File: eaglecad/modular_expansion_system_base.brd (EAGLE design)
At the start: 90.2 x 100 mm, 36 parts, among them IC1 74LS244N, IC2 74LS244N, IC3 74LS244N, IC4 SRAM, IC5 74LS30N, IC6 74LS30N, IC7 7805T, IC8 74LS00N, IC9 7805T, J1_ADDRESS_CON j1, J2_DATA_AND_POWER_CON j2, J3 interrupt_wait_block, SW1 100SP3T1B1M6QE

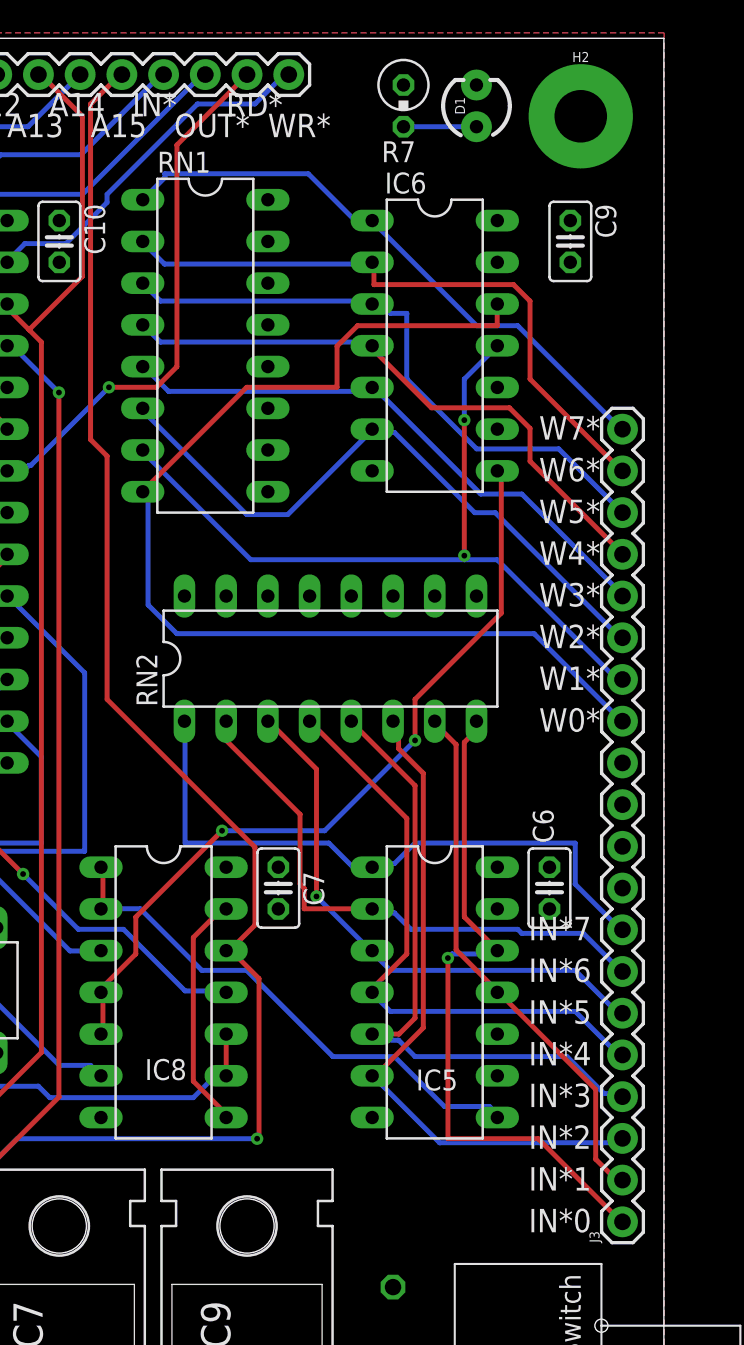
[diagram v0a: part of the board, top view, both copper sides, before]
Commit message: all three boards designed
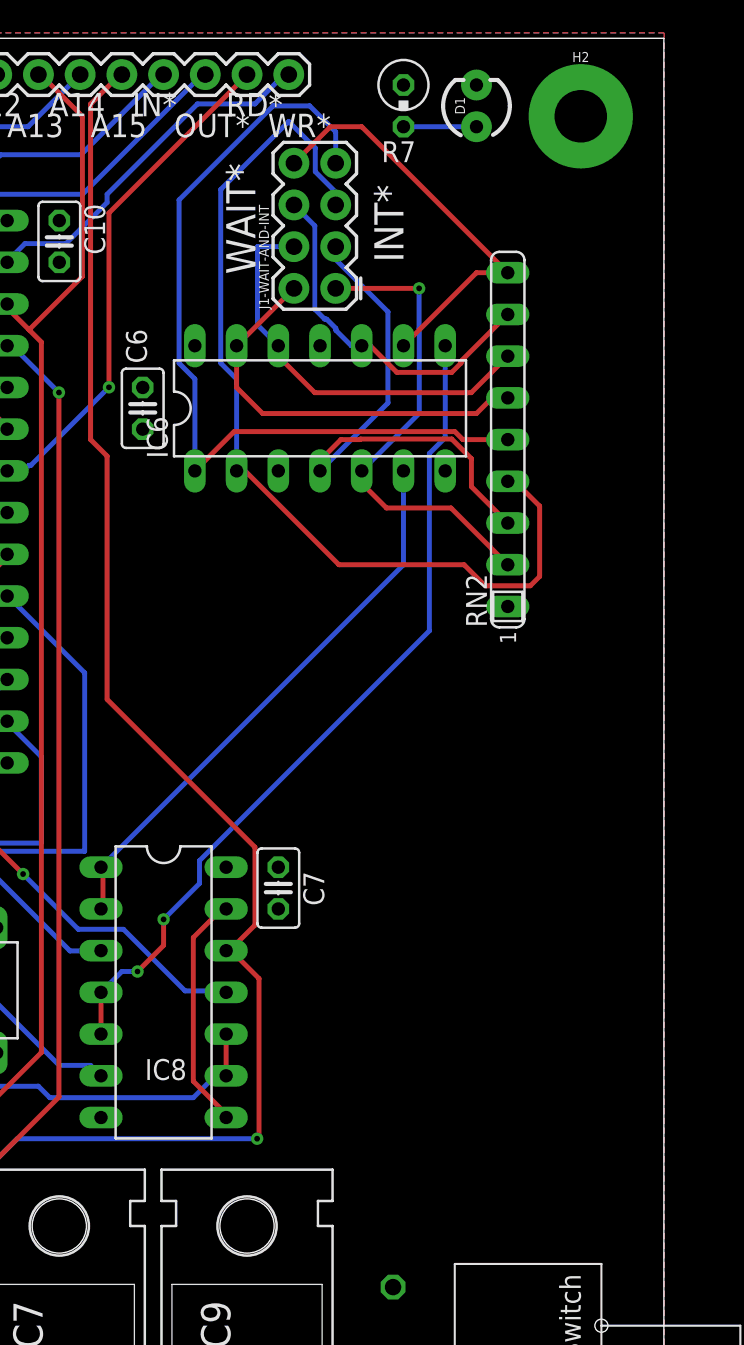
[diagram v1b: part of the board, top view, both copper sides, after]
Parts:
- removed C9: .1uf, rcl:C025-025X050
- removed IC5: 74LS30N, 74xx-us:DIL14
- removed J3: interrupt_wait_block, SparkFun-Connectors:1X20
- removed RN1: 4.7k, resistor-dil:DIL16
- added J1-WAIT-AND-INT: WAIT-AND-INT, SparkFun-Connectors:2X4
- IC6: value 74LS30N -> 74LS20N
- RN2: device resistor-dil:DIL16 -> resistor-sil:SIL9
- moved C6 38.3 mm to (58.4, 77.5)
- moved RN2 17.2 mm to (80.6, 75.6), turned to 90 degrees
- moved IC6 7.96 mm to (69.2, 77.5), turned to 0 degrees
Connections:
- removed net INT*0: IC5.12, J3.1, RN2.8
- removed net INT*1: IC5.11, J3.2, RN2.7
- removed net INT*2: IC5.6, J3.3, RN2.6
- removed net INT*3: IC5.5, J3.4, RN2.5
- removed net INT*4: IC5.4, J3.5, RN2.4
- removed net INT*5: IC5.3, J3.6, RN2.3
- removed net INT*6: IC5.2, J3.7, RN2.2
- removed net INT*7: IC5.1, J3.8, RN2.1
- removed net N$21: IC6.3, J3.18, RN1.3
- removed net WAIT*0: IC6.12, J3.13, RN1.8
- removed net WAIT*1: IC6.11, J3.14, RN1.7
- removed net WAIT*2: IC6.6, J3.15, RN1.6
- removed net WAIT*3: IC6.5, J3.16, RN1.5
- removed net WAIT*5: IC6.4, J3.17, RN1.4
- removed net WAIT*6: IC6.2, J3.19, RN1.2
- removed net WAIT*7: IC6.1, J3.20, RN1.1
- new net INT0*: IC6.5, J1-WAIT-AND-INT.1, RN2.2
- new net INT1*: IC6.4, J1-WAIT-AND-INT.3, RN2.3
- new net INT2*: IC6.2, J1-WAIT-AND-INT.5, RN2.4
- new net INT3*: IC6.1, J1-WAIT-AND-INT.7, RN2.5
- new net WAIT0*: IC6.13, J1-WAIT-AND-INT.2, RN2.6
- new net WAIT1*: IC6.12, J1-WAIT-AND-INT.4, RN2.7
- new net WAIT2*: IC6.10, J1-WAIT-AND-INT.6, RN2.8
- new net WAIT3*: IC6.9, J1-WAIT-AND-INT.8, RN2.9
- net GND: no longer C9.2, IC5.7
- net INT: now also IC6.6; no longer IC5.8
- net VCC: now also RN2.1; no longer C9.1, IC5.14, RN1.10, RN1.11, RN1.12, RN1.13, RN1.14, RN1.15, RN1.16, RN1.9, RN2.10, RN2.11, RN2.12, RN2.13, RN2.14, RN2.15, RN2.16, RN2.9
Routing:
- net WAIT*0: track 67.5 -> 0.00 mm
- net INT2*: track 0.00 -> 58.1 mm
- net INT3*: track 0.00 -> 51.6 mm
- net WAIT*1: track 48.9 -> 0.00 mm, vias 2 -> 0
- net INT*0: track 42.1 -> 0.00 mm, vias 1 -> 0
- net INT*2: track 40.8 -> 0.00 mm
- net INT*3: track 39.5 -> 0.00 mm
- net WAIT*2: track 39.4 -> 0.00 mm
- net INT*7: track 39.0 -> 0.00 mm
- net WAIT*6: track 38.6 -> 0.00 mm
- net N$21: track 37.3 -> 0.00 mm
- net INT*4: track 36.7 -> 0.00 mm
- net WAIT*7: track 36.4 -> 0.00 mm
- net WAIT*5: track 36.3 -> 0.00 mm
- net WAIT*3: track 35.3 -> 0.00 mm
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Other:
- board text added: "INT*"
- board text added: "WAIT*"
- board text removed: "IN*0"
- board text removed: "IN*1"
- board text removed: "IN*2"
- board text removed: "IN*3"
- board text removed: "IN*4"
- board text removed: "IN*5"
- board text removed: "IN*6"
- board text removed: "IN*7"
- board text removed: "W0*"
- board text removed: "W1*"
- board text removed: "W2*"
- board text removed: "W3*"
- board text removed: "W4*"
- board text removed: "W5*"
- board text removed: "W6*"
- board text removed: "W7*"
